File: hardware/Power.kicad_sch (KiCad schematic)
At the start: 1 part

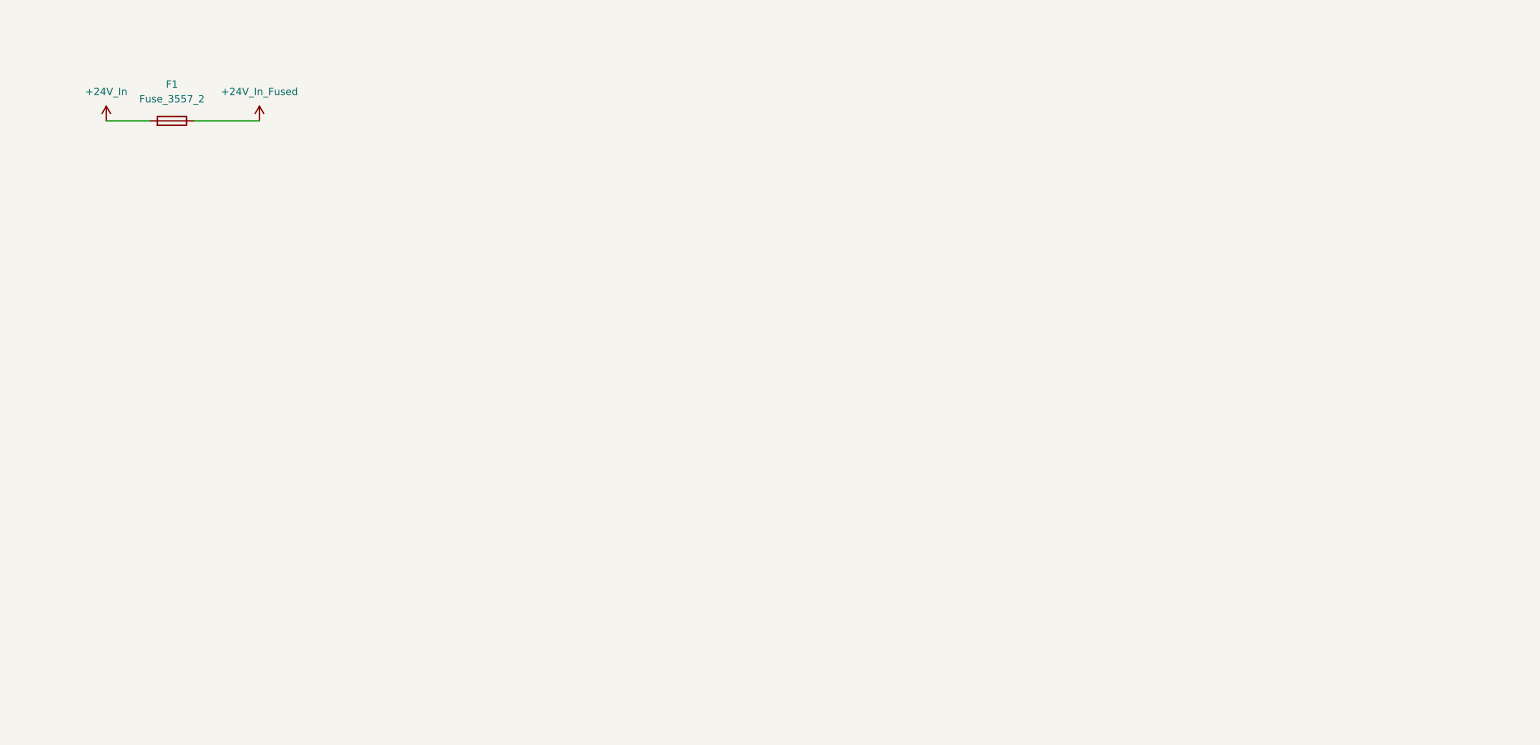
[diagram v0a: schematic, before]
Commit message: added more stuff wip
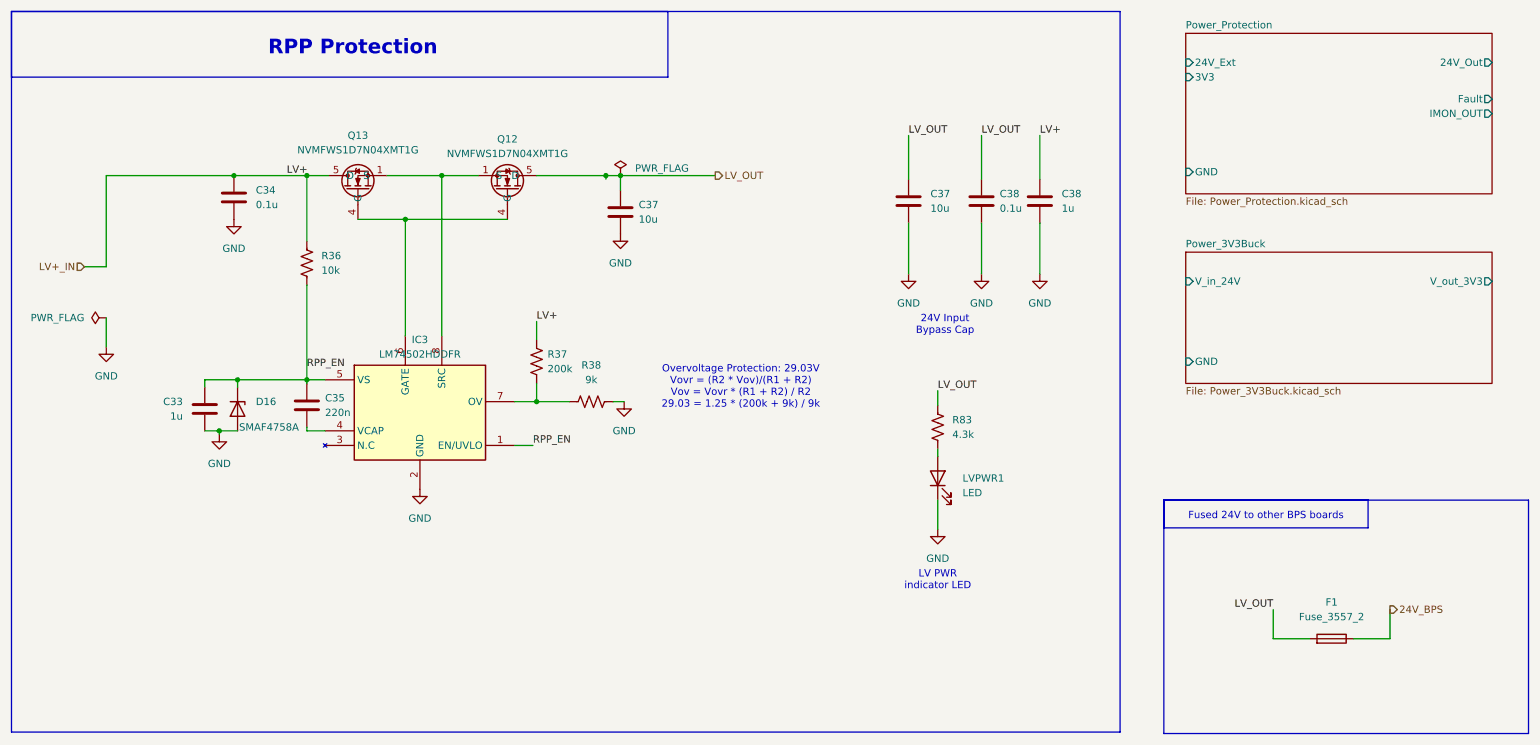
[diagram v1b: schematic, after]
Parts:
- added C33, C38: 1u, Capacitor_SMD:C_0603_1608Metric, symbol Device:C
- added C34, C38: 0.1u, Capacitor_SMD:C_0603_1608Metric, symbol Device:C
- added C35: 220n, Capacitor_SMD:C_0603_1608Metric, symbol Device:C
- added C37 (x2): 10u, Capacitor_SMD:C_0805_2012Metric, symbol Device:C
- added D16: SMAF4758A, UTSVT_Passives:SODFL4724X108N, symbol Device:D_Zener
- added IC3: LM74502HDDFR, UTSVT_Power:SOT65P280X110-8N, symbol UTSVT_ICs:LM74502HDDFR
- added LVPWR1: LED, LED_SMD:LED_0603_1608Metric, symbol Device:LED
- added Q12, Q13: NVMFWS1D7N04XMT1G, UTSVT_Power:NVMFWS3D0P04M8LT1G, symbol UTSVT_Power:NVMFWS1D7N04XMT1G
- added R36: 10k, Resistor_SMD:R_0603_1608Metric, symbol Device:R_US
- added R37: 200k, Resistor_SMD:R_0603_1608Metric, symbol Device:R_US
- added R38: 9k, Resistor_SMD:R_0603_1608Metric, symbol Device:R_US
- added R83: 4.3k, Resistor_SMD:R_0603_1608Metric, symbol Device:R_US
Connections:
- net +24V_In renamed LV_OUT
- net LV_OUT: now also C37.1, C37.1, C38.1, Q12.5 (D), Q12.6 (D), Q12.7 (D), Q12.8 (D), Q12.9 (D), R83.1
- net +24V_In_Fused renamed 24V_BPS
- new net: C35.2, IC3.4 (VCAP)
- new net: IC3.6 (GATE), Q12.4 (G), Q13.4 (G)
- new net: IC3.7 (OV), R37.2, R38.1
- new net: IC3.8 (SRC), Q12.1 (S), Q12.2 (S), Q12.3 (S), Q13.1 (S), Q13.2 (S), Q13.3 (S)
- new net: LVPWR1.2 (A), R83.2
- new net GND: C33.1, C34.2, C37.2, C37.2, C38.2, C38.2, D16.2 (A), IC3.2 (GND), LVPWR1.1 (K), R38.2
- new net LV+_IN: C34.1, C38.1, Q13.5 (D), Q13.6 (D), Q13.7 (D), Q13.8 (D), Q13.9 (D), R36.1, R37.1
- new net RPP_EN: C33.2, C35.1, D16.1 (K), IC3.1 (EN/UVLO), IC3.5 (VS), R36.2
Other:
- added sheet Power_3V3Buck (Power_3V3Buck.kicad_sch)
- added sheet Power_Protection (Power_Protection.kicad_sch)
- note added: "24V Input Bypass Cap"
- note added: "Fused 24V to other BPS boards"
- note added: "LV PWR indicator LED"
- note added: "Overvoltage Protection: 29.03V Vovr = (R2 * Vov)/(R1 + R2) Vov = Vovr * (R1 + R2) / R2 29.03 = 1.25 * (200k + 9k) / 9k"
- note added: "RPP Protection"
- moved on the sheet: F1
